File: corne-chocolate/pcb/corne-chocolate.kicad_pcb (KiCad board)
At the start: 2 copper layers, 133.8 x 91.4 mm, 99 parts, among them J1 MJ-4PP-9, J2 OLED, J3 LED, J6 Conn_01x04, P1 i2c-pin, P2 i2c-pin, SW1 SW_PUSH, SW10 SW_PUSH, SW11 SW_PUSH, SW12 SW_PUSH, SW13 SW_PUSH, SW14 SW_PUSH, SW15 SW_PUSH, SW16 SW_PUSH, SW17 SW_PUSH, SW18 SW_PUSH, SW19 SW_PUSH, SW2 SW_PUSH, SW20 SW_PUSH, SW21 SW_PUSH, SW3 SW_PUSH, SW4 SW_PUSH, SW5 SW_PUSH, SW6 SW_PUSH, SW7 SW_PUSH, SW8 SW_PUSH, SW9 SW_PUSH, U1 ProMicro

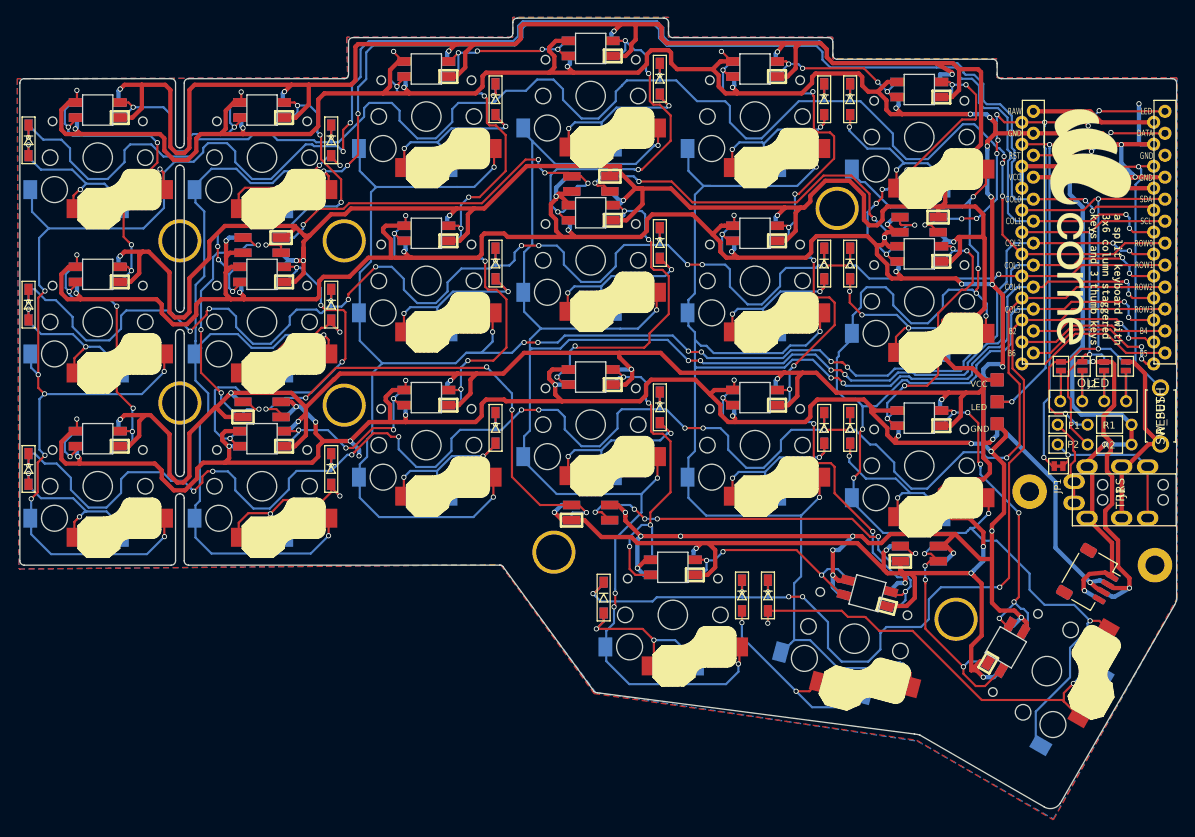
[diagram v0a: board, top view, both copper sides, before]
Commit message: ProMicro USB-C
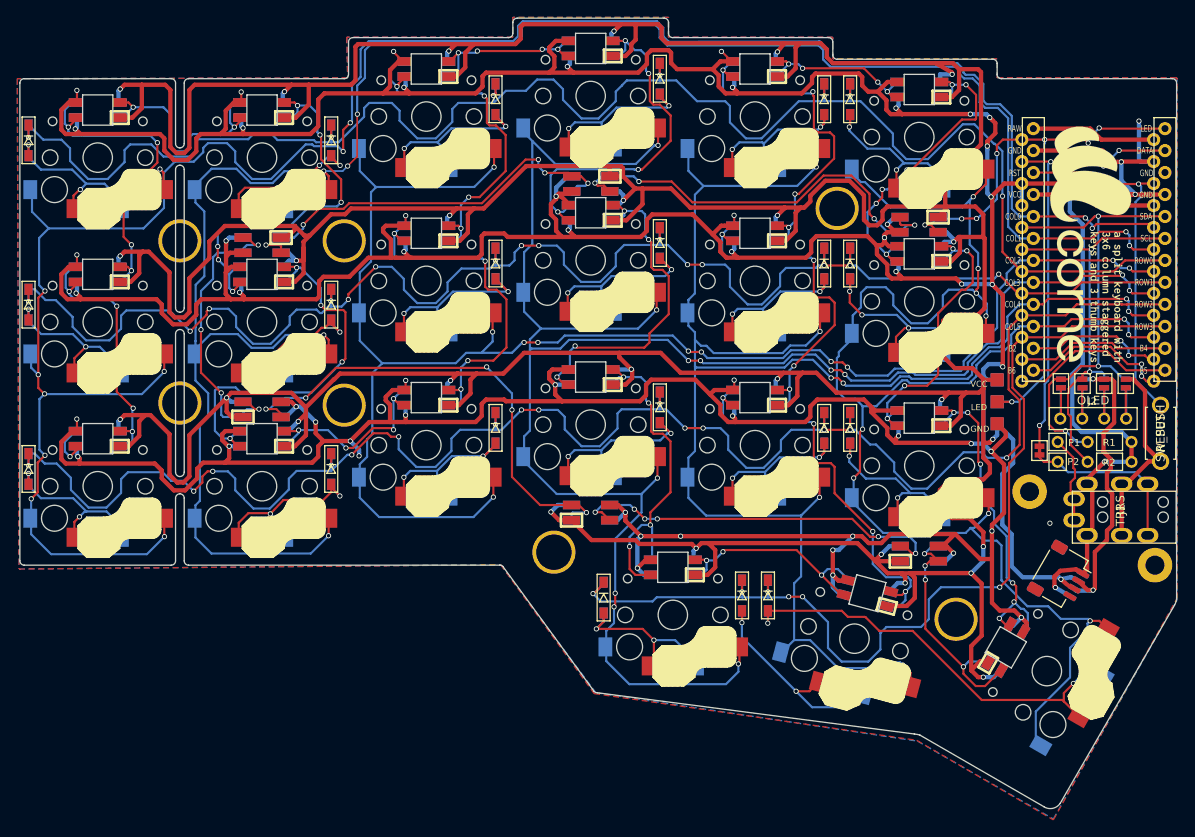
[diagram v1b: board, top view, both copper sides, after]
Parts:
- moved J6 3.39 mm to (181.4, 125.5)
- moved JP1 2.84 mm to (178.9, 111.0), turned to -90 degrees
- moved G*** 2.00 mm to (184.7, 87.2)
- moved G*** 2.00 mm to (184.0, 87.0)
- moved J1 2.00 mm to (194.7, 118.7)
- moved J2 2.00 mm to (181.3, 107.3)
- moved JP2 2.00 mm to (188.9, 103.2)
- moved JP3 2.00 mm to (186.4, 103.2)
- moved JP4 2.00 mm to (183.9, 103.2)
- moved JP5 2.00 mm to (181.4, 103.2)
- moved JP6 2.00 mm to (188.9, 103.2)
- moved JP7 2.00 mm to (186.4, 103.2)
- moved JP8 2.00 mm to (183.9, 103.2)
- moved JP9 2.00 mm to (181.4, 103.2)
- moved P1 2.00 mm to (181.0, 110.0)
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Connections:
- J3 pad 3: VDD -> +5V
- J6 pad 3: VDD -> +5V
- L1 pad 4: VDD -> +5V
- L10 pad 4: VDD -> +5V
- L11 pad 4: VDD -> +5V
- L12 pad 4: VDD -> +5V
- L13 pad 4: VDD -> +5V
- L14 pad 4: VDD -> +5V
- L15 pad 4: VDD -> +5V
- L16 pad 4: VDD -> +5V
- L17 pad 4: VDD -> +5V
- L18 pad 4: VDD -> +5V
- L19 pad 4: VDD -> +5V
- L2 pad 4: VDD -> +5V
- L20 pad 4: VDD -> +5V
- L21 pad 4: VDD -> +5V
- L22 pad 4: VCC -> +5V
- L23 pad 4: VCC -> +5V
- L24 pad 4: VCC -> +5V
- L25 pad 4: VCC -> +5V
- L26 pad 4: VCC -> +5V
- L27 pad 4: VCC -> +5V
- L3 pad 4: VDD -> +5V
- L4 pad 4: VDD -> +5V
- L5 pad 4: VDD -> +5V
- L6 pad 4: VDD -> +5V
- L7 pad 4: VDD -> +5V
- L8 pad 4: VDD -> +5V
- L9 pad 4: VDD -> +5V
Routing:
- net +5V: track 0.00 -> 750.5 mm, vias 0 -> 28
- net VDD: track 750.0 -> 0.00 mm, vias 29 -> 0
- net Net-(J1-PadB): track 74.8 -> 20.0 mm, vias 5 -> 0
- net data: track 0.00 -> 51.0 mm, vias 0 -> 4
- net GND: track 791.8 -> 775.9 mm, vias 58 -> 59
- net LED: track 79.9 -> 74.4 mm, vias 10 -> 8
- net col2: track 193.4 -> 188.5 mm
- net OLED_PWR: track 38.5 -> 34.5 mm
- net VCC: track 80.0 -> 76.6 mm
- net col4: track 196.2 -> 193.3 mm
- net col3: track 224.8 -> 222.5 mm
- net row2: track 209.9 -> 207.9 mm
- net row3: track 119.2 -> 117.2 mm
- net row0: track 197.4 -> 199.2 mm, vias 9 -> 7
- net col0: track 255.1 -> 256.6 mm
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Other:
- board text added: "Corne Chocolate v2.1 PCB designed by foostan Wirelessed by Allen"
- board text removed: "Wireless Corne Chocolate v2.1 PCB designed by foostan modified by Allen"

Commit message: minor chagnes
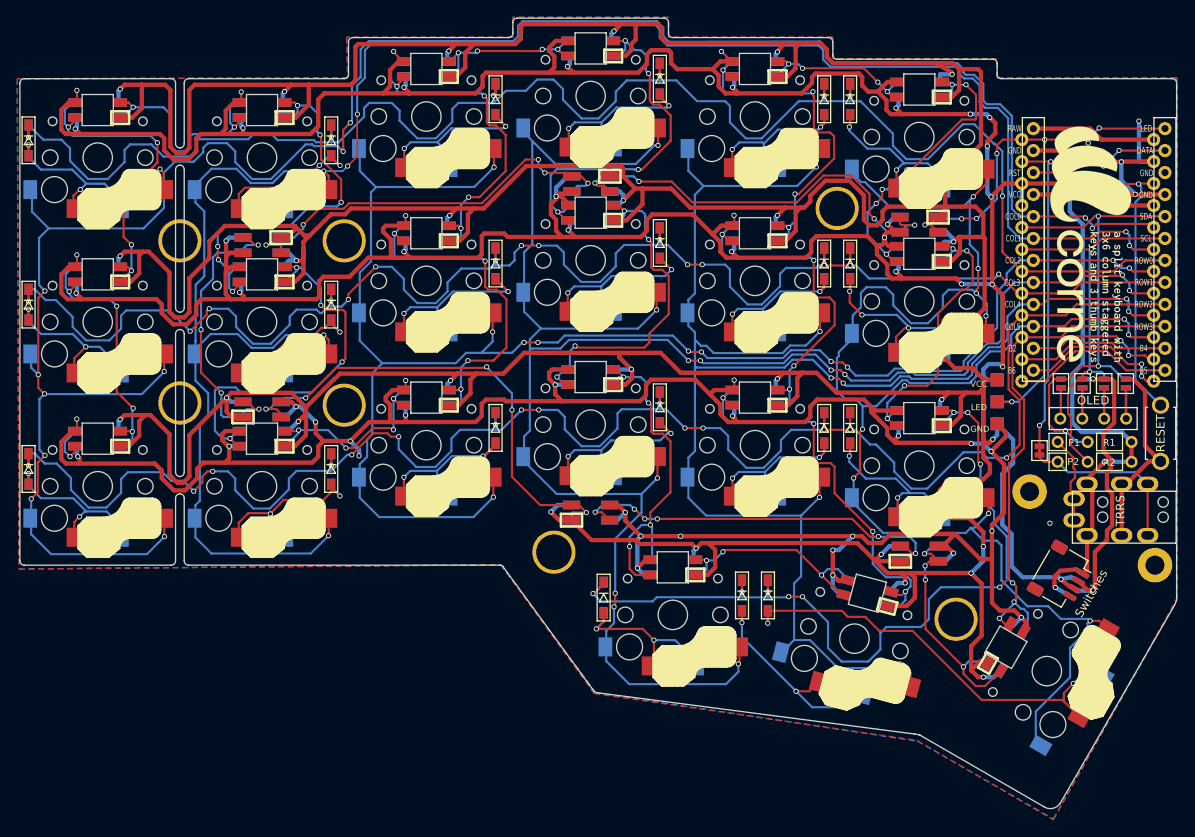
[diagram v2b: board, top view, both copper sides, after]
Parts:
- renumbered J6 to Switches
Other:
- board text added: "Corne Chocolate v2.1.2 PCB designed by foostan Wirelessed by Allen"
- board text removed: "Corne Chocolate v2.1 PCB designed by foostan Wirelessed by Allen"
- board text removed: "OLED"
